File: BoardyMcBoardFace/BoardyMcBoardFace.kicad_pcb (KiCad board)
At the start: 4 copper layers, 95 x 24 mm, 83 parts, among them J1 SMA, J2 ARM 10pin, J3 USB_B_Micro, SW1 SW_Push, U1 nRF24L01P, U2 STM32F103CBT6, U3 USBLC6-2SC6, U4 LM393, U5 AMS1117-5.0, U6 AMS1117-3.3, U7 USBLC6-2SC6, U8 USBLC6-2SC6, U9 TJA1051T-3, Y1 16MHz, Y2 16MHz

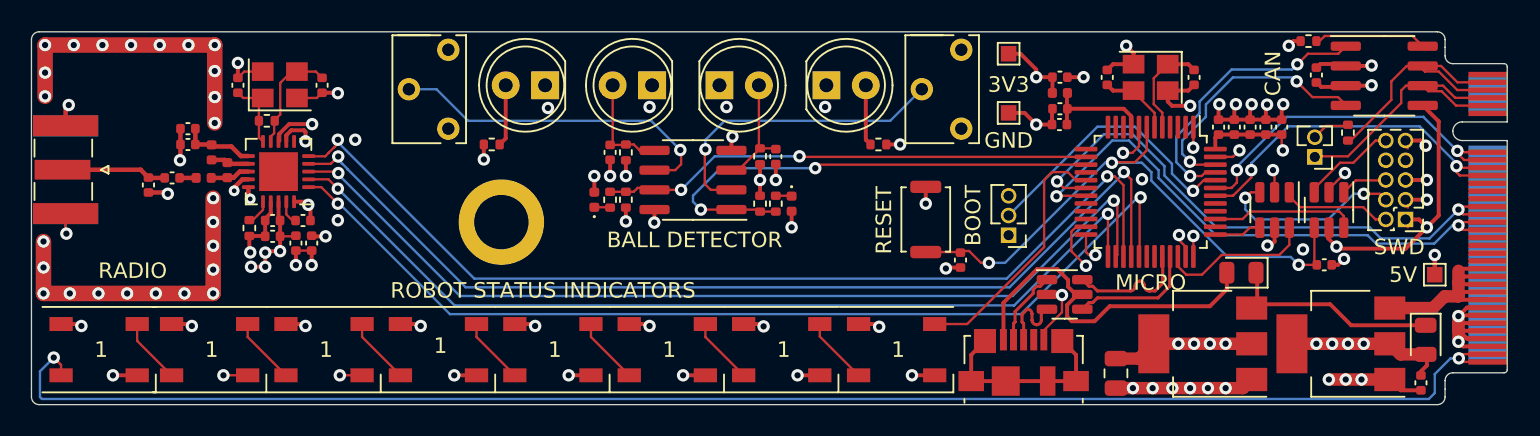
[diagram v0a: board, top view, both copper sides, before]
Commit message: fix comments
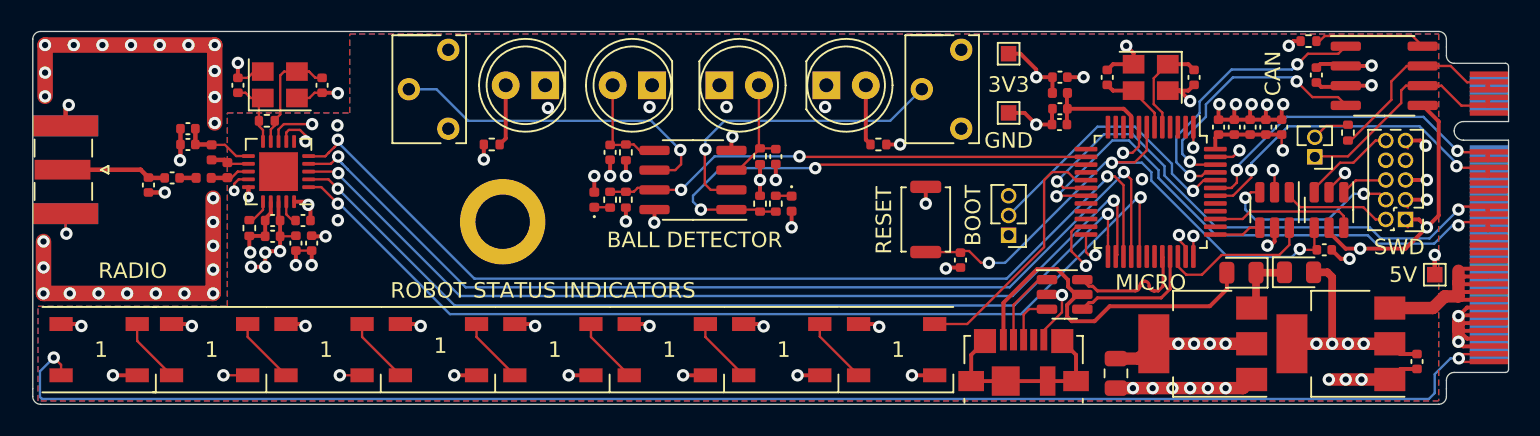
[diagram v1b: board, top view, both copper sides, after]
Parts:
- moved D5 9.24 mm to (189.9, 114.1), turned to 0 degrees
- moved C26 1.40 mm to (197.5, 119.9)
- moved C20 0.97 mm to (191.5, 112.7)
- moved U$1 0.09 mm to (203.4, 110.6)
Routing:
- net Net-(D5-Pad1): track 14.3 -> 4.23 mm
- net /CAN_H: track 17.2 -> 12.8 mm
- net /CAN_L: track 18.6 -> 14.5 mm
- net +5V: track 15.3 -> 18.9 mm
- net /I2C1_SCL: track 23.6 -> 21.6 mm
- net /I2C1_SDA: track 23.3 -> 21.5 mm
- net /USB_CONN_DP: track 4.85 -> 3.28 mm
- net /DRBL_PWM_1: track 37.0 -> 35.5 mm
- net /DRBL_PWM_2: track 36.8 -> 35.3 mm
- net /NRST: track 37.8 -> 36.8 mm
- net +3V3: track 75.4 -> 74.9 mm, vias 36 -> 35
- added copper zone on B.Cu, net GND
- added copper zone on F.Cu, net GND
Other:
- outline, holes or cut-outs redrawn

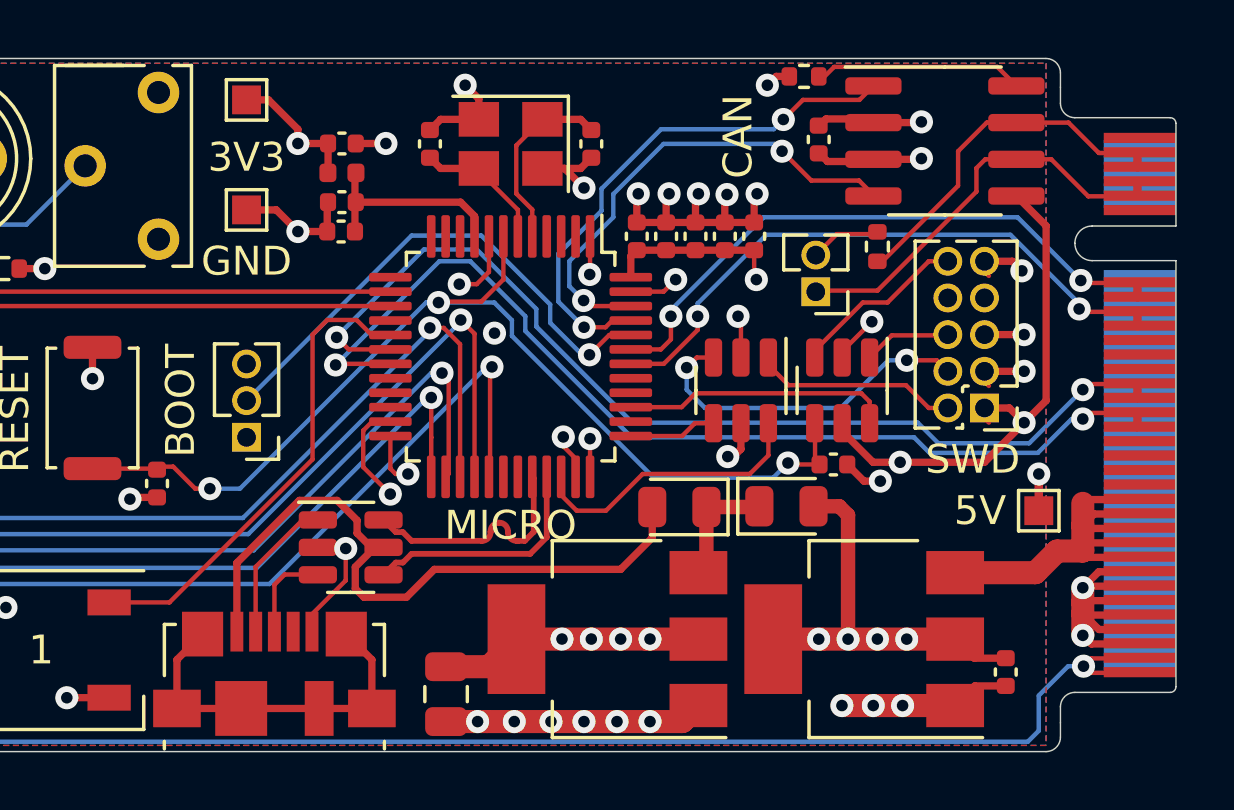
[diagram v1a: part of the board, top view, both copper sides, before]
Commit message: wip
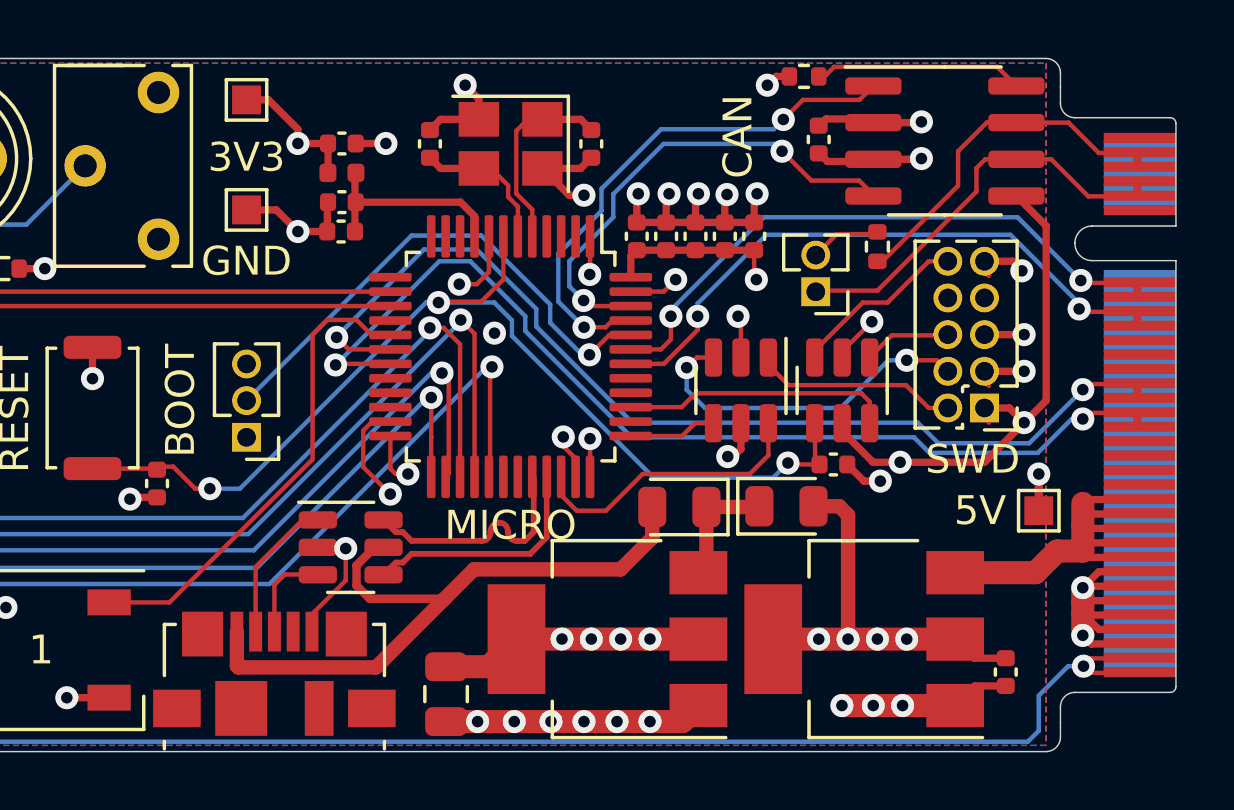
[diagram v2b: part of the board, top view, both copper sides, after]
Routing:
- net unconnected-(J3-Pad6): track 12.6 -> 0.00 mm
- net VBUS: track 22.9 -> 23.6 mm

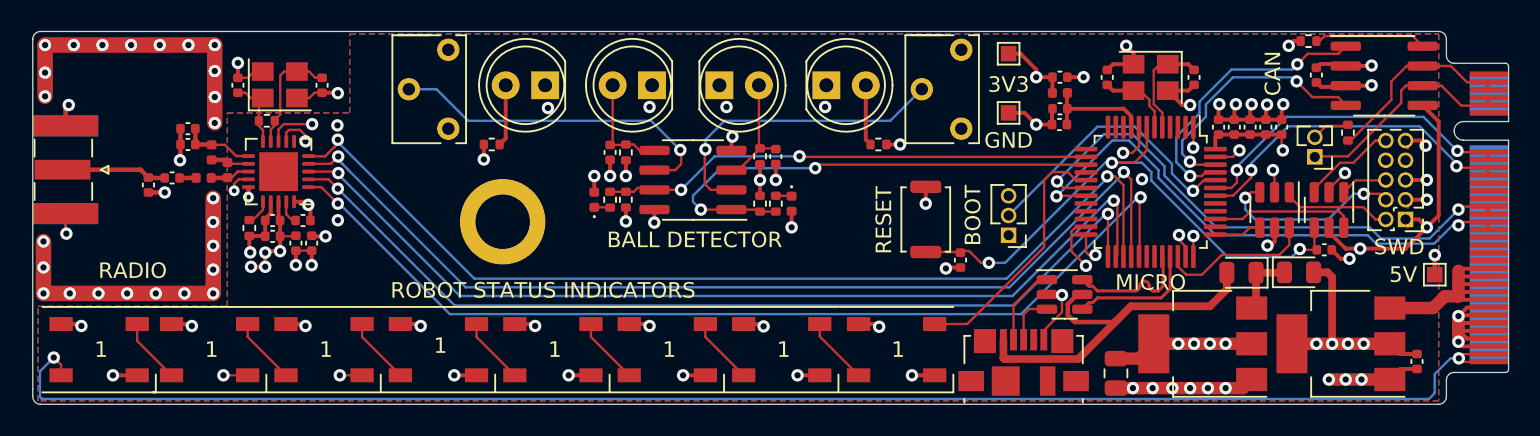
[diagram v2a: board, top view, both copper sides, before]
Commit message: wip
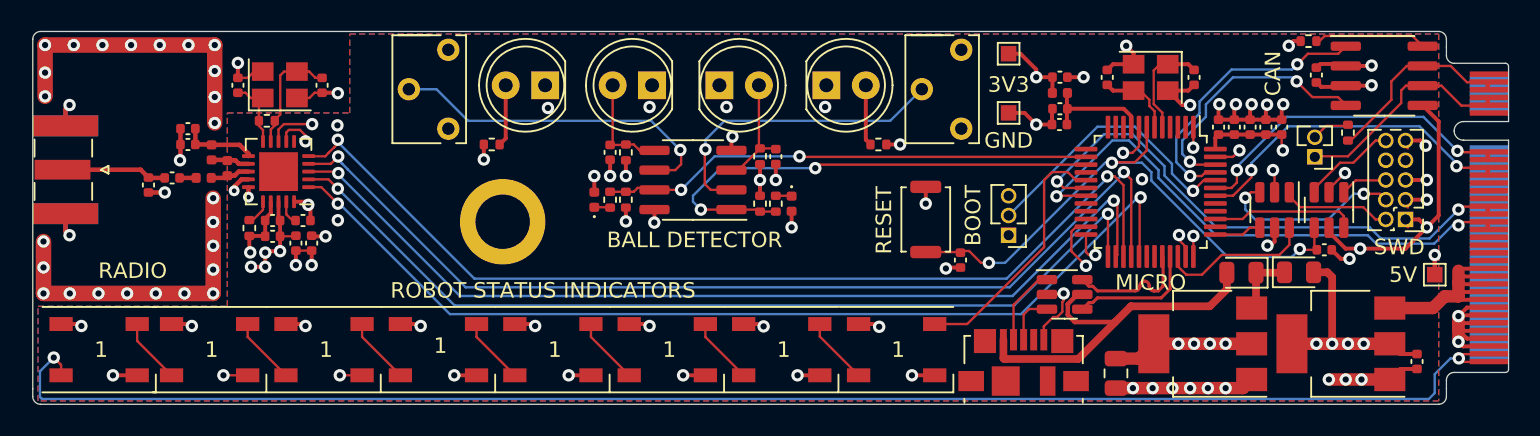
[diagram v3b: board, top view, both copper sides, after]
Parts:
- moved L2 0.13 mm to (120.9, 107.4)
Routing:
- net GND: track 162.4 -> 163.1 mm

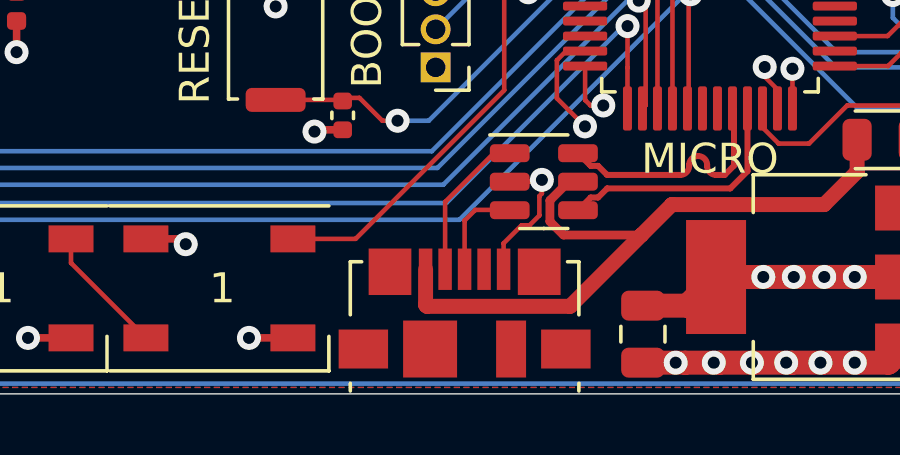
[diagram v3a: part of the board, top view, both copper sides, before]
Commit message: wip
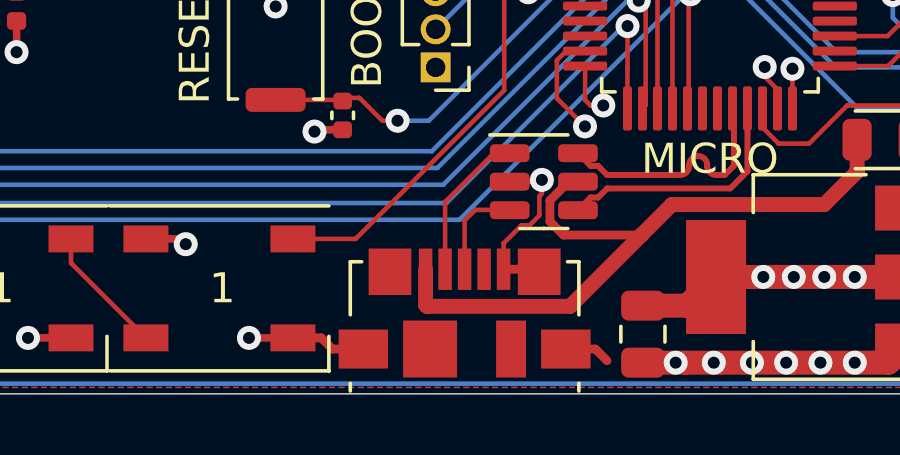
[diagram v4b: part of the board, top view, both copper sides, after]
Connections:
- J3 pad 6: unconnected-(J3-Pad6) -> GND
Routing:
- net GND: track 163.1 -> 168.3 mm
